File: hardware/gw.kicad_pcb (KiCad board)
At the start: 4 copper layers, 47 x 32.9 mm, 21 parts, among them J1 USB_OTG, J2 Conn_01x04, U1 ESP-12F, U2 Ai-Thinker-Ra-02, U3 AMS1117-3.3

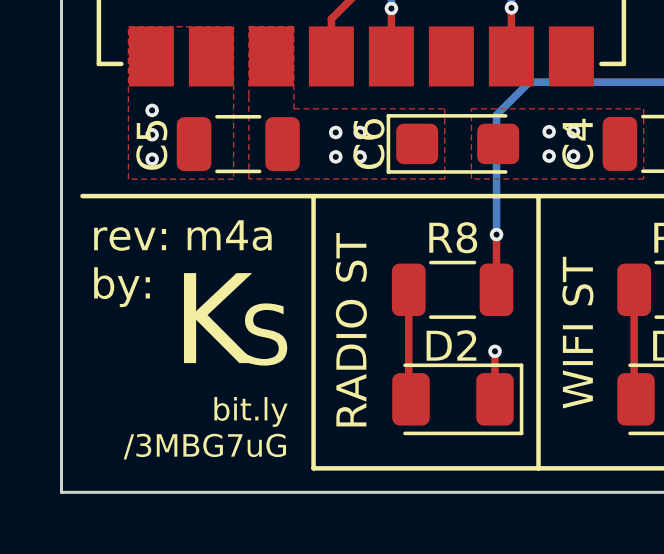
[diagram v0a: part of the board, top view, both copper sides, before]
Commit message: Fix rev
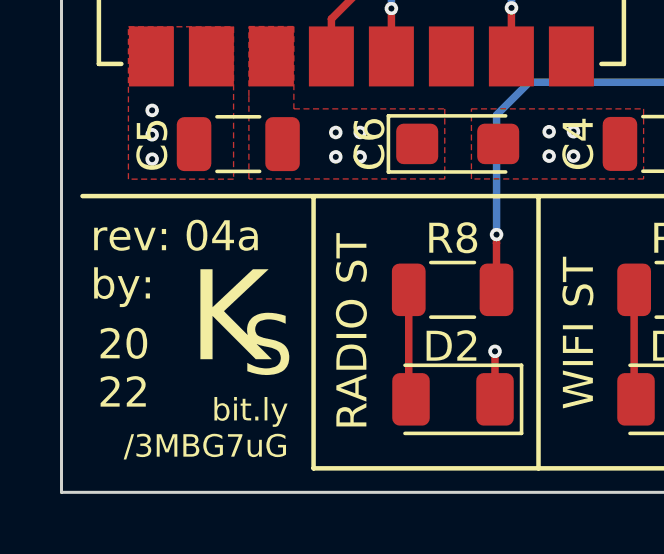
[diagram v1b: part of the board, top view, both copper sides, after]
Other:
- board text added: "20 22"
- board text added: "rev: 04a by:"
- board text removed: "rev: m4a by:"
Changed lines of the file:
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@@
     (effects (font (size 0.75 0.75) (thickness 0.15)) (justify right))
   )
-  (gr_text "S" (at 86.106 70.612) (layer "F.SilkS")
+  (gr_text "S" (at 86.175 70.925) (layer "F.SilkS")
     (effects (font (size 2 2) (thickness 0.2)))
   )
@@
     (effects (font (size 0.75 0.75) (thickness 0.15)) (justify right))
   )
-  (gr_text "rev: m4a\nby:" (at 80.264 68.072) (layer "F.SilkS")
+  (gr_text "rev: 04a\nby:" (at 80.264 68.072) (layer "F.SilkS")
     (effects (font (size 1 1) (thickness 0.2)) (justify left))
   )
-  (gr_text "K" (at 84.328 70.104) (layer "F.SilkS")
+  (gr_text "K" (at 84.875 69.975) (layer "F.SilkS")
     (effects (font (size 3 3) (thickness 0.2)))
   )
@@
     (effects (font (size 0.75 0.75) (thickness 0.15)) (justify right))
   )
+  (gr_text "20\n22" (at 81.375 71.675) (layer "F.SilkS")
+    (effects (font (size 1 1) (thickness 0.2)))
+  )
   (dimension (type aligned) (layer "B.Cu")
